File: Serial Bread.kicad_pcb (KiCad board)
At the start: 2 copper layers, 26 x 32 mm, 22 parts, among them J1 TYPE-C-31-M-12, J2 Conn_02x04_Top_Bottom, U1 CH340C, U2 AP2112K-3.3

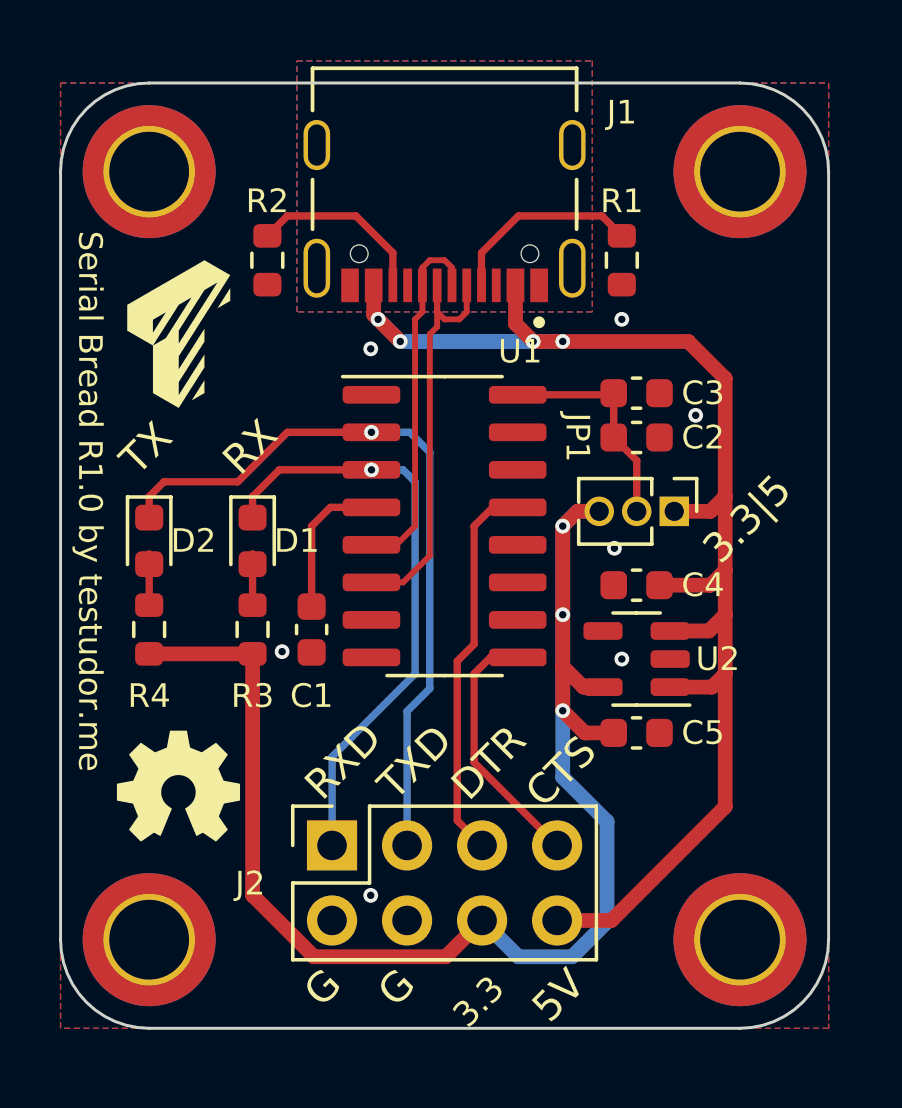
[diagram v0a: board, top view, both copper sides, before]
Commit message: Initial commit R1.1
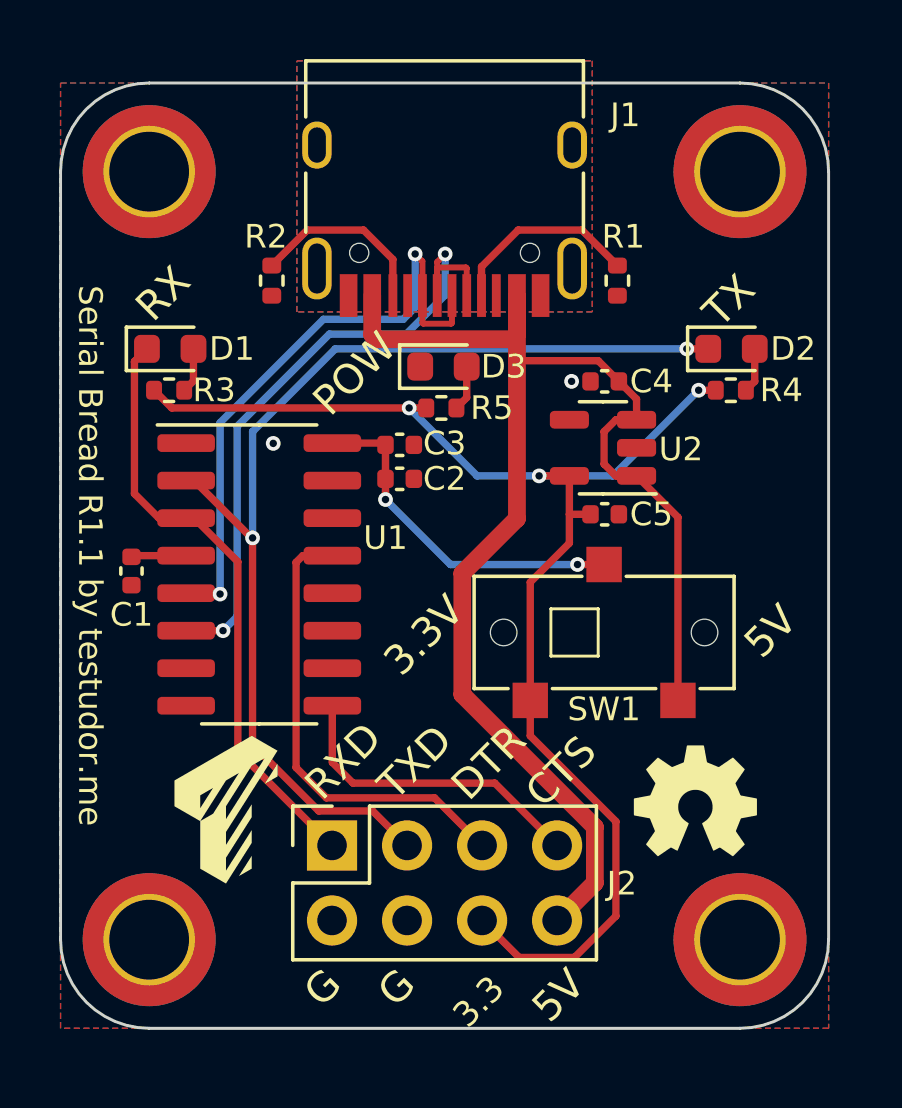
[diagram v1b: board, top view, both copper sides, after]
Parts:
- removed JP1: Jumper_3_Open, Connector_PinHeader_1.27mm:PinHeader_1x03_P1.27mm_Vertical
- added D3: LED RED, LED_SMD:LED_0603_1608Metric, F.Cu at (160.0, 85.6)
- added R5: 1k, Resistor_SMD:R_0402_1005Metric, F.Cu at (159.9, 87.0)
- added SW1: SW_SPDT, Custom_Switches:CL-SB-12B-02T, F.Cu at (165.4, 94.6)
- C1, C2, C3, C4, C5: footprint Capacitor_SMD:C_0603_1608Metric -> Capacitor_SMD:C_0402_1005Metric
- J1: value TYPE-C-31-M-12 -> USB_C_Receptacle_USB2.0; footprint SnapEDA Library:HRO_TYPE-C-31-M-12 -> Connector_USB:USB_C_Receptacle_HRO_TYPE-C-31-M-12
- R1, R2, R3, R4: footprint Resistor_SMD:R_0603_1608Metric -> Resistor_SMD:R_0402_1005Metric
- moved R4 21.3 mm to (169.7, 86.4), turned to 0 degrees
- moved D2 20.8 mm to (169.7, 85.0), turned to 0 degrees
- moved REF** 17.5 mm to (168.5, 100.5)
- moved REF** 16.2 mm to (152.6, 100.6)
- moved R3 8.58 mm to (150.7, 86.4), turned to 0 degrees
- moved C3 8.21 mm to (158.5, 88.2)
- moved C2 8.14 mm to (158.5, 89.4)
- moved C5 7.48 mm to (165.4, 90.6)
- moved U2 7.24 mm to (165.4, 88.3)
- moved D1 7.07 mm to (150.7, 85.0), turned to 0 degrees
- moved C4 6.98 mm to (165.4, 86.1)
- moved U1 6.48 mm to (153.7, 92.6)
- moved C1 6.41 mm to (149.4, 92.5)
- moved J1 1.05 mm to (160.0, 79.2)
- moved R1 0.71 mm to (165.8, 82.7)
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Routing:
- net /TXD: track 25.0 -> 36.6 mm, vias 1 -> 2
- net /D+: track 12.4 -> 21.4 mm, vias 0 -> 2
- net /D-: track 14.6 -> 23.0 mm, vias 0 -> 2
- net +3.3V: track 52.9 -> 46.0 mm
- net VCC: track 7.60 -> 11.9 mm, vias 0 -> 2
- net Net-(U1-V3): track 5.01 -> 1.81 mm
- net /DTR: track 13.1 -> 15.7 mm
- net /CTS: track 8.68 -> 10.7 mm
- net Net-(D3-A): track 0.00 -> 1.54 mm
- net +5V: track 48.3 -> 49.1 mm, vias 4 -> 0
- net /RXD: vias 1 -> 0
- net GND: vias 7 -> 2
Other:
- board text added: "3.3V"
- board text added: "POW"
- board text added: "Serial Bread R1.1 by testudor.me"
- board text removed: "3.3|5"
- board text removed: "Serial Bread R1.0 by testudor.me"
